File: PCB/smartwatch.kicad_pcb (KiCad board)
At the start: 4 copper layers, 36 x 36 mm, 45 parts, among them J1 Serial wire/Charging, J2 Battery input, J3 Conn_01x15, J4 Conn_01x03, J5 USB_B_Micro, SW1 SW_SPDT, U1 STM32L432KBUx, U2 LSM6DS3, U3 W25Q128JVPIQ, U4 TP4056, U5 LT1761-3.3, U6 INA3221, U8 USBLC6-2SC6, X2 20Mhz, Y2 LSE 32khz

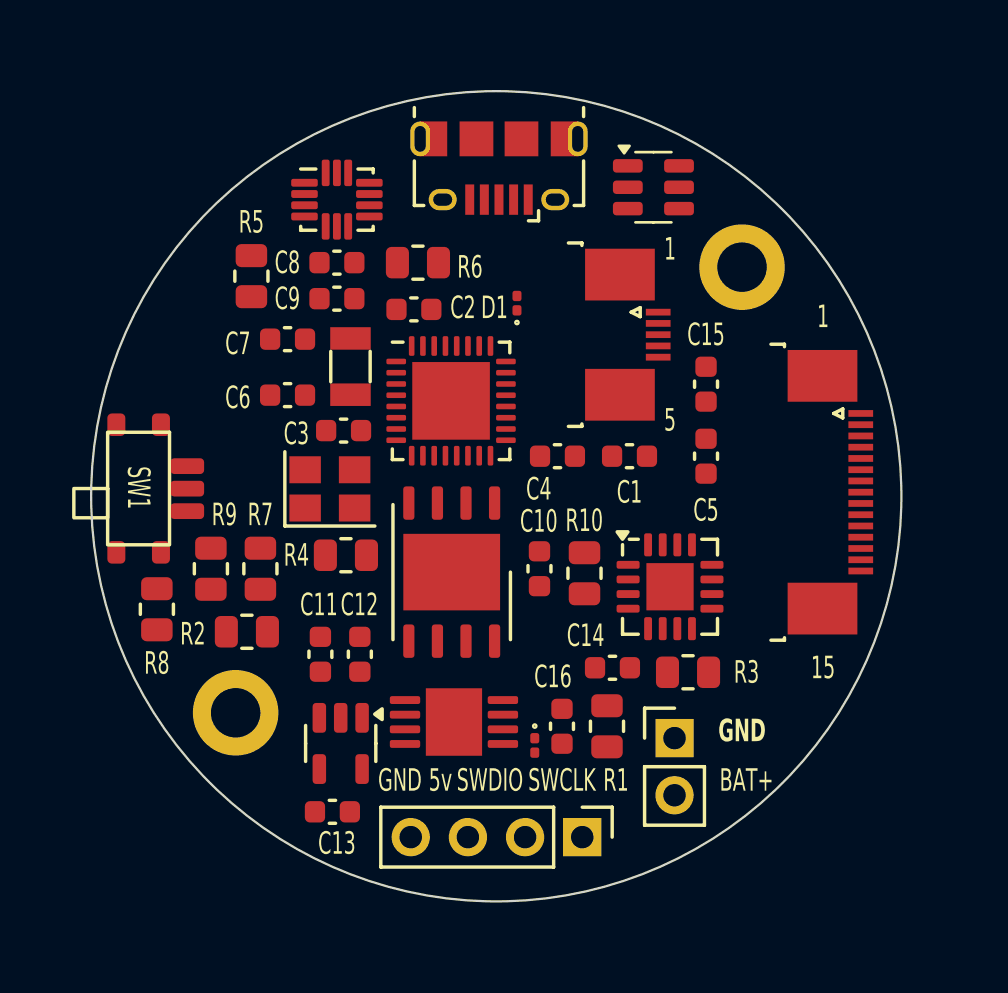
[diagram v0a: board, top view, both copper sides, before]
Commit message: pcb done
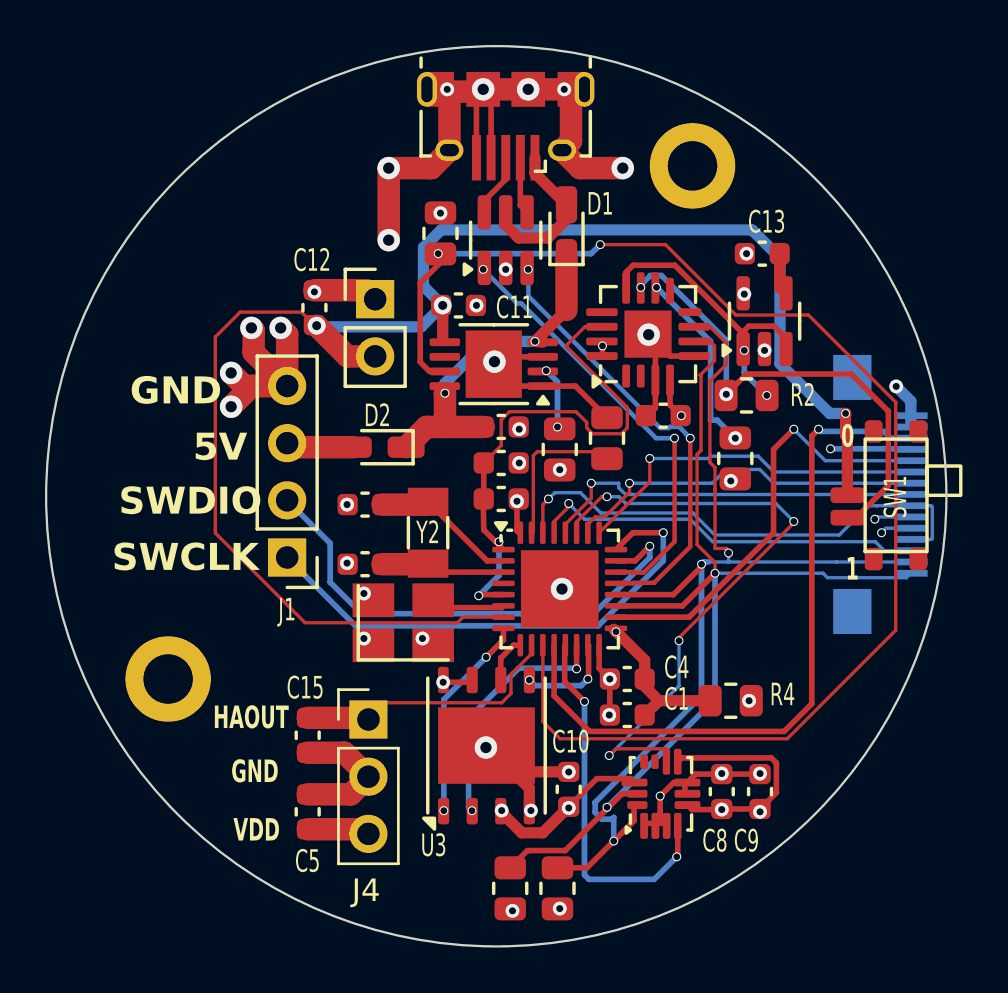
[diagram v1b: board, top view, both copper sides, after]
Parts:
- removed R8: [Jumper], Resistor_SMD:R_0805_2012Metric
- removed R9: 4.7k, Resistor_SMD:R_0805_2012Metric
- D1, D2: footprint Diode_SMD:D_0201_0603Metric -> Diode_SMD:D_0603_1608Metric
- J3: footprint Connector_FFC-FPC:TE_1-1734839-5_1x15-1MP_P0.5mm_Horizontal -> MyButtons:FPC-SMD_15P-P0.50_KH-FG0.5-H2.0-15P-SMT; moved to B.Cu
- J4: footprint Connector_FFC-FPC:TE_0-1734839-5_1x05-1MP_P0.5mm_Horizontal -> Connector_PinHeader_2.54mm:PinHeader_1x03_P2.54mm_Vertical
- moved C13 31.3 mm to (169.3, 83.2)
- moved U2 30.1 mm to (164.8, 107.2), turned to 90 degrees
- moved R5 29.5 mm to (158.1, 111.4)
- moved C8 29.1 mm to (167.5, 107.1), turned to -90 degrees
- moved C9 28.9 mm to (169.2, 107.1), turned to -90 degrees
- moved R6 28.5 mm to (160.2, 111.4), turned to 90 degrees
- moved U5 26.6 mm to (169.4, 86.2), turned to 90 degrees
- moved R2 24.6 mm to (168.6, 89.5)
- moved C5 23.7 mm to (149.1, 108.0)
- moved J2 23.6 mm to (152.1, 85.2)
- moved C15 23.6 mm to (149.1, 104.6)
- moved J4 20.6 mm to (151.8, 103.9), turned to 0 degrees
- moved SW1 18.5 mm to (167.6, 94.7), turned to 90 degrees
- moved R4 18.3 mm to (167.9, 103.1), turned to 0 degrees
- moved J1 18.1 mm to (148.2, 96.7), turned to 180 degrees
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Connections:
- C1 pad 2: VDD -> VDDSHUNTL
- C2 pad 2: VDD -> VDDSHUNTL
- C3 pad 2: VDD -> VDDSHUNTL
- C4 pad 2: VDD -> VDDSHUNTL
- J1 pad 1: Net-(J1-Pin_1) -> SWCLK
- J1 pad 2: Net-(J1-Pin_2) -> SWDIO
- J3 pad 12: TP_RST -> LCD_RST
- J3 pad 9: RST -> LCD_RST
- R2 pad 1: BATSHUNTH -> BATSHUNTL
- R4 pad 1: VDD -> VDDSHUNTL
- SW1 pad 1: BATSHUNTH -> BATSHUNTL
- U1 pad 1: VDD -> VDDSHUNTL
- U1 pad 17: VDD -> VDDSHUNTL
- U1 pad 21: USB_DM -> USB_D-
- U1 pad 22: USB_DP -> USB_D+
- U1 pad 30: TP_RST -> LCD_RST
- U1 pad 5: VDD -> VDDSHUNTL
- U6 pad 11: BATSHUNTH -> BATSHUNTL
- U6 pad 14: VDD -> VDDSHUNTL
- U8 pad 1: Net-(J5-D+) -> USB_D+
- U8 pad 3: Net-(J5-D-) -> USB_D-
- U8 pad 4: USB_DM -> Net-(J5-D-)
- U8 pad 6: USB_DP -> Net-(J5-D+)
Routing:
- net GND: track 0.00 -> 85.5 mm, vias 0 -> 36
- net BAT: track 0.00 -> 71.1 mm, vias 0 -> 3
- net CHARGE: track 0.00 -> 61.5 mm, vias 0 -> 2
- net I2C1_SDA: track 0.00 -> 46.2 mm, vias 0 -> 3
- net I2C1_SCL: track 0.00 -> 45.0 mm, vias 0 -> 2
- net VDDSHUNTL: track 0.00 -> 37.5 mm, vias 0 -> 3
- net LEDA: track 0.00 -> 31.5 mm, vias 0 -> 1
- net VDD: track 0.00 -> 29.6 mm, vias 0 -> 17
- net GYRO_INT2: track 0.00 -> 28.2 mm, vias 0 -> 4
- net SWCLK: track 0.00 -> 22.8 mm, vias 0 -> 1
- net SWDIO: track 0.00 -> 22.5 mm, vias 0 -> 1
- net LCD_RST: track 0.00 -> 22.5 mm, vias 0 -> 1
- net BATSHUNTL: track 0.00 -> 21.6 mm, vias 0 -> 2
- net USB_D-: track 0.00 -> 19.8 mm, vias 0 -> 2
- net USB_D+: track 0.00 -> 19.4 mm, vias 0 -> 2
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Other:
- board size 36 x 36 mm -> 40 x 40 mm
- board text added: "0"
- board text added: "5V"
- board text added: "HAOUT"
- board text added: "VDD"
- board text removed: "15"
- board text removed: "5"
- board text removed: "5v"
- board text removed: "BAT+"
